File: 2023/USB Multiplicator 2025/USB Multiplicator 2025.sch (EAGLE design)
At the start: 9 parts, among them X1 USB-A

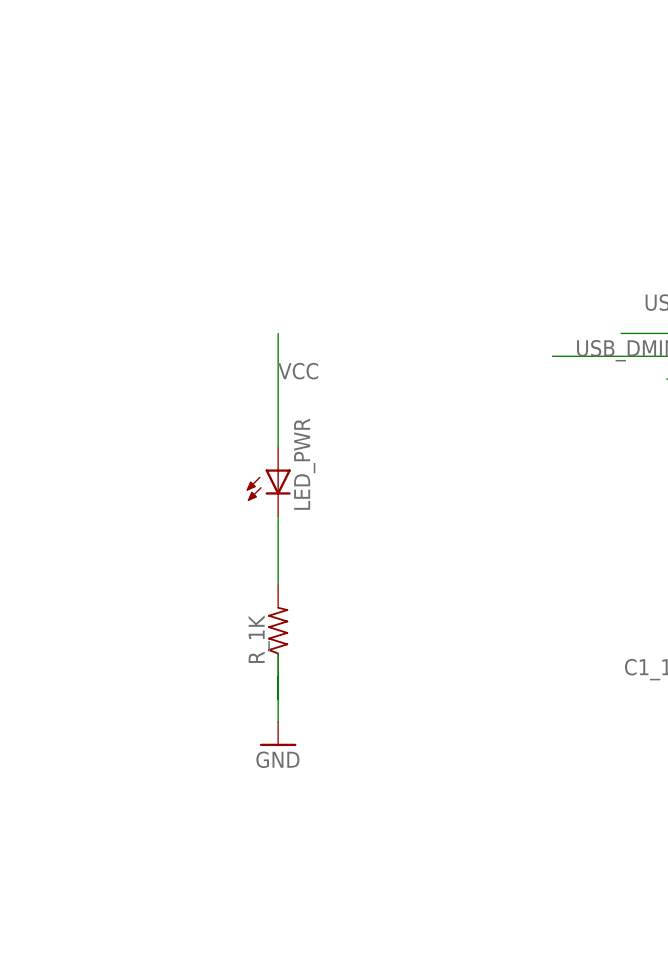
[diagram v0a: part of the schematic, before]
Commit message: Update...
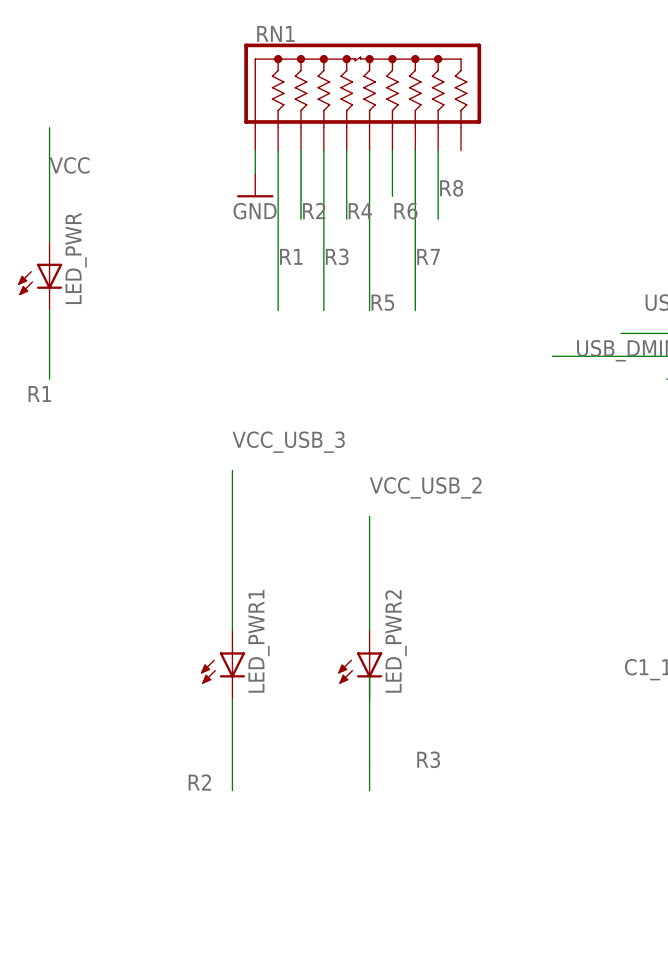
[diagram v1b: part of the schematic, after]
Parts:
- removed R_1K: (no value), adafruit:R-US_R1206
- added LED_PWR1, LED_PWR2: (no value), adafruit:LEDSMT1206
- added RN1: (no value), resistor-sip:4610X
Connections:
- removed net N$5: LED_PWR.C, R_1K.2
- new net R1: LED_PWR.C, RN1.2
- new net R2: LED_PWR1.C, RN1.3
- new net R3: LED_PWR2.C, RN1.4
- new net R4: RN1.5
- new net R5: RN1.6
- new net R6: RN1.7
- new net R7: RN1.8
- new net R8: RN1.9
- net GND: now also RN1.1; no longer R_1K.1
- net VCC_USB_2: now also LED_PWR2.A
- net VCC_USB_3: now also LED_PWR1.A
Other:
- moved on the sheet: LED_PWR
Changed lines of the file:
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@@
 <part name="GND6" library="supply1" deviceset="GND" device=""/>
 <part name="LED_PWR" library="adafruit" deviceset="LED" device="SMT1206"/>
-<part name="R_1K" library="adafruit" deviceset="R-US_" device="R1206"/>
-<part name="GND7" library="supply1" deviceset="GND" device=""/>
 <part name="USB_OUT_WITH_DATA_1" library="STUNTAZ" deviceset="USB" device=""/>
 <part name="GND2" library="supply1" deviceset="GND" device=""/>
@@
 <part name="S2" library="adafruit" deviceset="EG1218" device="S"/>
 <part name="S1" library="adafruit" deviceset="EG1218" device="S"/>
+<part name="LED_PWR2" library="adafruit" deviceset="LED" device="SMT1206"/>
+<part name="LED_PWR1" library="adafruit" deviceset="LED" device="SMT1206"/>
+<part name="RN1" library="resistor-sip" deviceset="4610X" device=""/>
+<part name="GND9" library="supply1" deviceset="GND" device=""/>
 </parts>
 <sheets>
@@
 <attribute name="VALUE" x="35.56" y="66.04" size="1.778" layer="96"/>
 </instance>
-<instance part="LED_PWR" gate="G$1" x="-12.7" y="99.06" smashed="yes">
-<attribute name="NAME" x="-9.144" y="94.488" size="1.778" layer="95" rot="R90"/>
-<attribute name="VALUE" x="-6.985" y="94.488" size="1.778" layer="96" rot="R90"/>
-</instance>
-<instance part="R_1K" gate="G$1" x="-12.7" y="81.28" smashed="yes" rot="R90">
-<attribute name="NAME" x="-14.1986" y="77.47" size="1.778" layer="95" rot="R90"/>
-<attribute name="VALUE" x="-9.398" y="77.47" size="1.778" layer="96" rot="R90"/>
-</instance>
-<instance part="GND7" gate="1" x="-12.7" y="68.58" smashed="yes">
-<attribute name="VALUE" x="-15.24" y="66.04" size="1.778" layer="96"/>
+<instance part="LED_PWR" gate="G$1" x="-38.1" y="121.92" smashed="yes">
+<attribute name="NAME" x="-34.544" y="117.348" size="1.778" layer="95" rot="R90"/>
+<attribute name="VALUE" x="-32.385" y="117.348" size="1.778" layer="96" rot="R90"/>
 </instance>
 <instance part="USB_OUT_WITH_DATA_1" gate="G$1" x="55.88" y="104.14" smashed="yes"/>
@@
 <attribute name="NAME" x="108.585" y="49.53" size="1.778" layer="95" rot="R180"/>
 <attribute name="VALUE" x="103.505" y="52.07" size="1.778" layer="96" rot="R180"/>
+</instance>
+<instance part="LED_PWR2" gate="G$1" x="-2.54" y="78.74" smashed="yes">
+<attribute name="NAME" x="1.016" y="74.168" size="1.778" layer="95" rot="R90"/>
+<attribute name="VALUE" x="3.175" y="74.168" size="1.778" layer="96" rot="R90"/>
+</instance>
+<instance part="LED_PWR1" gate="G$1" x="-17.78" y="78.74" smashed="yes">
+<attribute name="NAME" x="-14.224" y="74.168" size="1.778" layer="95" rot="R90"/>
+<attribute name="VALUE" x="-12.065" y="74.168" size="1.778" layer="96" rot="R90"/>
+</instance>
+<instance part="RN1" gate="G$1" x="-2.54" y="139.7" smashed="yes">
+<attribute name="NAME" x="-15.24" y="146.685" size="1.778" layer="95"/>
+<attribute name="VALUE" x="0" y="146.685" size="1.778" layer="96"/>
+</instance>
+<instance part="GND9" gate="1" x="-15.24" y="129.54" smashed="yes">
+<attribute name="VALUE" x="-17.78" y="127" size="1.778" layer="96"/>
 </instance>
 </instances>
@@
 </segment>
 <segment>
-<pinref part="R_1K" gate="G$1" pin="1"/>
-<pinref part="GND7" gate="1" pin="GND"/>
-<wire x1="-12.7" y1="76.2" x2="-12.7" y2="73.66" width="0.1524" layer="91"/>
-<wire x1="-12.7" y1="73.66" x2="-12.7" y2="71.12" width="0.1524" layer="91"/>
-<wire x1="-12.7" y1="78.74" x2="-12.7" y2="73.66" width="0.1524" layer="91"/>
-</segment>
-<segment>
 <pinref part="USB_OUT_WITH_DATA_1" gate="G$1" pin="GND"/>
 <pinref part="GND2" gate="1" pin="GND"/>
@@
 <wire x1="81.28" y1="81.28" x2="86.36" y2="81.28" width="0.1524" layer="91"/>
 </segment>
+<segment>
+<pinref part="RN1" gate="G$1" pin="1"/>
+<pinref part="GND9" gate="1" pin="GND"/>
+<wire x1="-15.24" y1="134.62" x2="-15.24" y2="132.08" width="0.1524" layer="91"/>
+</segment>
 </net>
 <net name="VCC" class="0">
@@
 <segment>
 <pinref part="LED_PWR" gate="G$1" pin="A"/>
-<wire x1="-12.7" y1="101.6" x2="-12.7" y2="114.3" width="0.1524" layer="91"/>
-<label x="-12.7" y="109.22" size="1.778" layer="95"/>
+<wire x1="-38.1" y1="124.46" x2="-38.1" y2="137.16" width="0.1524" layer="91"/>
+<label x="-38.1" y="132.08" size="1.778" layer="95"/>
 </segment>
 <segment>
@@
 </segment>
 </net>
-<net name="N$5" class="0">
-<segment>
-<pinref part="LED_PWR" gate="G$1" pin="C"/>
-<pinref part="R_1K" gate="G$1" pin="2"/>
-<wire x1="-12.7" y1="93.98" x2="-12.7" y2="86.36" width="0.1524" layer="91"/>
-</segment>
-</net>
 <net name="USB_DPLUS" class="0">
 <segment>
@@
 <label x="50.8" y="83.82" size="1.778" layer="95"/>
 </segment>
+<segment>
+<pinref part="LED_PWR2" gate="G$1" pin="A"/>
+<wire x1="-2.54" y1="81.28" x2="-2.54" y2="93.98" width="0.1524" layer="91"/>
+<label x="-2.54" y="96.52" size="1.778" layer="95"/>
+</segment>
 </net>
 <net name="VCC_USB_3" class="0">
@@
 <label x="86.36" y="53.34" size="1.778" layer="95"/>
 </segment>
-</net>
+<segment>
+<pinref part="LED_PWR1" gate="G$1" pin="A"/>
+<wire x1="-17.78" y1="81.28" x2="-17.78" y2="99.06" width="0.1524" layer="91"/>
+<label x="-17.78" y="101.6" size="1.778" layer="95"/>
+</segment>
+</net>
+<net name="R1" class="0">
+<segment>
+<pinref part="RN1" gate="G$1" pin="2"/>
+<wire x1="-12.7" y1="134.62" x2="-12.7" y2="116.84" width="0.1524" layer="91"/>
+<label x="-12.7" y="121.92" size="1.778" layer="95"/>
+</segment>
+<segment>
+<pinref part="LED_PWR" gate="G$1" pin="C"/>
+<wire x1="-38.1" y1="116.84" x2="-38.1" y2="109.22" width="0.1524" layer="91"/>
+<label x="-40.64" y="106.68" size="1.778" layer="95"/>
+</segment>
+</net>
+<net name="R2" class="0">
+<segment>
+<pinref part="RN1" gate="G$1" pin="3"/>
+<wire x1="-10.16" y1="134.62" x2="-10.16" y2="127" width="0.1524" layer="91"/>
+<label x="-10.16" y="127" size="1.778" layer="95"/>
+</segment>
+<segment>
+<pinref part="LED_PWR1" gate="G$1" pin="C"/>
+<wire x1="-17.78" y1="63.5" x2="-17.78" y2="73.66" width="0.1524" layer="91"/>
+<label x="-22.86" y="63.5" size="1.778" layer="95"/>
+</segment>
+</net>
+<net name="R3" class="0">
+<segment>
+<pinref part="RN1" gate="G$1" pin="4"/>
+<wire x1="-7.62" y1="134.62" x2="-7.62" y2="116.84" width="0.1524" layer="91"/>
+<label x="-7.62" y="121.92" size="1.778" layer="95"/>
+</segment>
+<segment>
+<pinref part="LED_PWR2" gate="G$1" pin="C"/>
+<wire x1="-2.54" y1="73.66" x2="-2.54" y2="66.04" width="0.1524" layer="91"/>
+<wire x1="-2.54" y1="66.04" x2="-2.54" y2="63.5" width="0.1524" layer="91"/>
+<wire x1="-2.54" y1="76.2" x2="-2.54" y2="73.66" width="0.1524" layer="91"/>
+<label x="2.54" y="66.04" size="1.778" layer="95"/>
+</segment>
+</net>
+<net name="R4" class="0">
+<segment>
+<pinref part="RN1" gate="G$1" pin="5"/>
+<wire x1="-5.08" y1="134.62" x2="-5.08" y2="127" width="0.1524" layer="91"/>
+<label x="-5.08" y="127" size="1.778" layer="95"/>
+</segment>
+</net>
+<net name="R5" class="0">
+<segment>
+<pinref part="RN1" gate="G$1" pin="6"/>
+<wire x1="-2.54" y1="134.62" x2="-2.54" y2="116.84" width="0.1524" layer="91"/>
+<label x="-2.54" y="116.84" size="1.778" layer="95"/>
+</segment>
+</net>
+<net name="R6" class="0">
+<segment>
+<pinref part="RN1" gate="G$1" pin="7"/>
+<wire x1="0" y1="134.62" x2="0" y2="129.54" width="0.1524" layer="91"/>
+<label x="0" y="127" size="1.778" layer="95"/>
+</segment>
+</net>
+<net name="R7" class="0">
+<segment>
+<pinref part="RN1" gate="G$1" pin="8"/>
+<wire x1="2.54" y1="134.62" x2="2.54" y2="116.84" width="0.1524" layer="91"/>
+<label x="2.54" y="121.92" size="1.778" layer="95"/>
+</segment>
+</net>
+<net name="R8" class="0">
+<segment>
+<pinref part="RN1" gate="G$1" pin="9"/>
+<wire x1="5.08" y1="134.62" x2="5.08" y2="127" width="0.1524" layer="91"/>
+<label x="5.08" y="129.54" size="1.778" layer="95"/>
+</segment>
+</net>
